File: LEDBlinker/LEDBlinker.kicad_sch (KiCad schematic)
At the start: 19 parts, among them J1 Conn_01x02_Pin, Q1 2N7000, Q2 2N7000, Q3 2N7000, SW1 SW_SPDT, U1 ICM7555xP

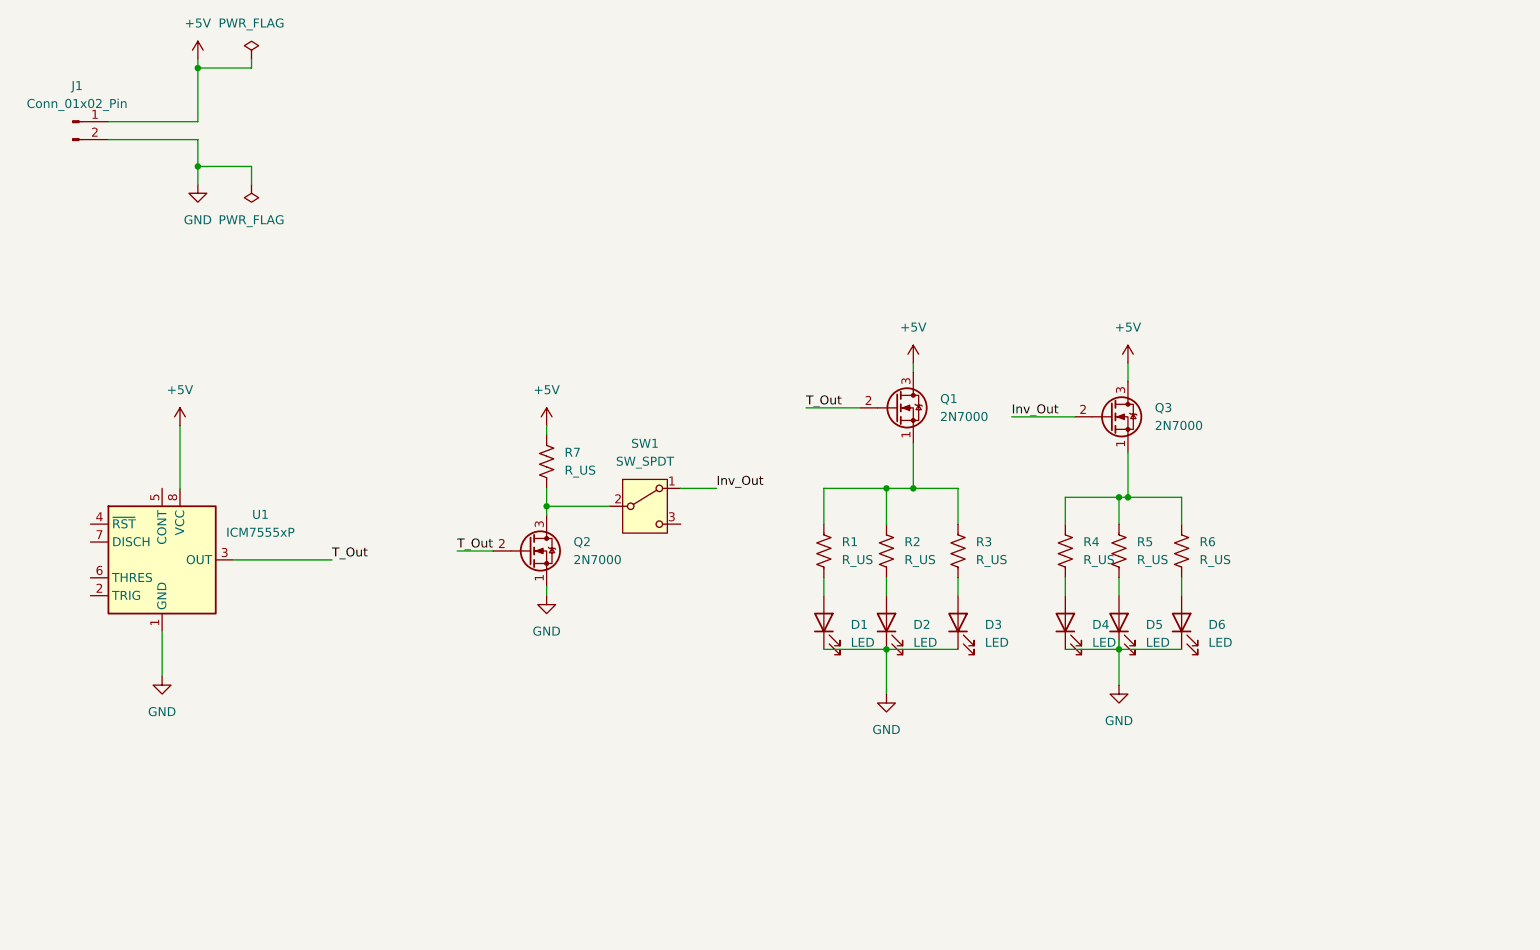
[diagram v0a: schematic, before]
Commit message: Initial Commit
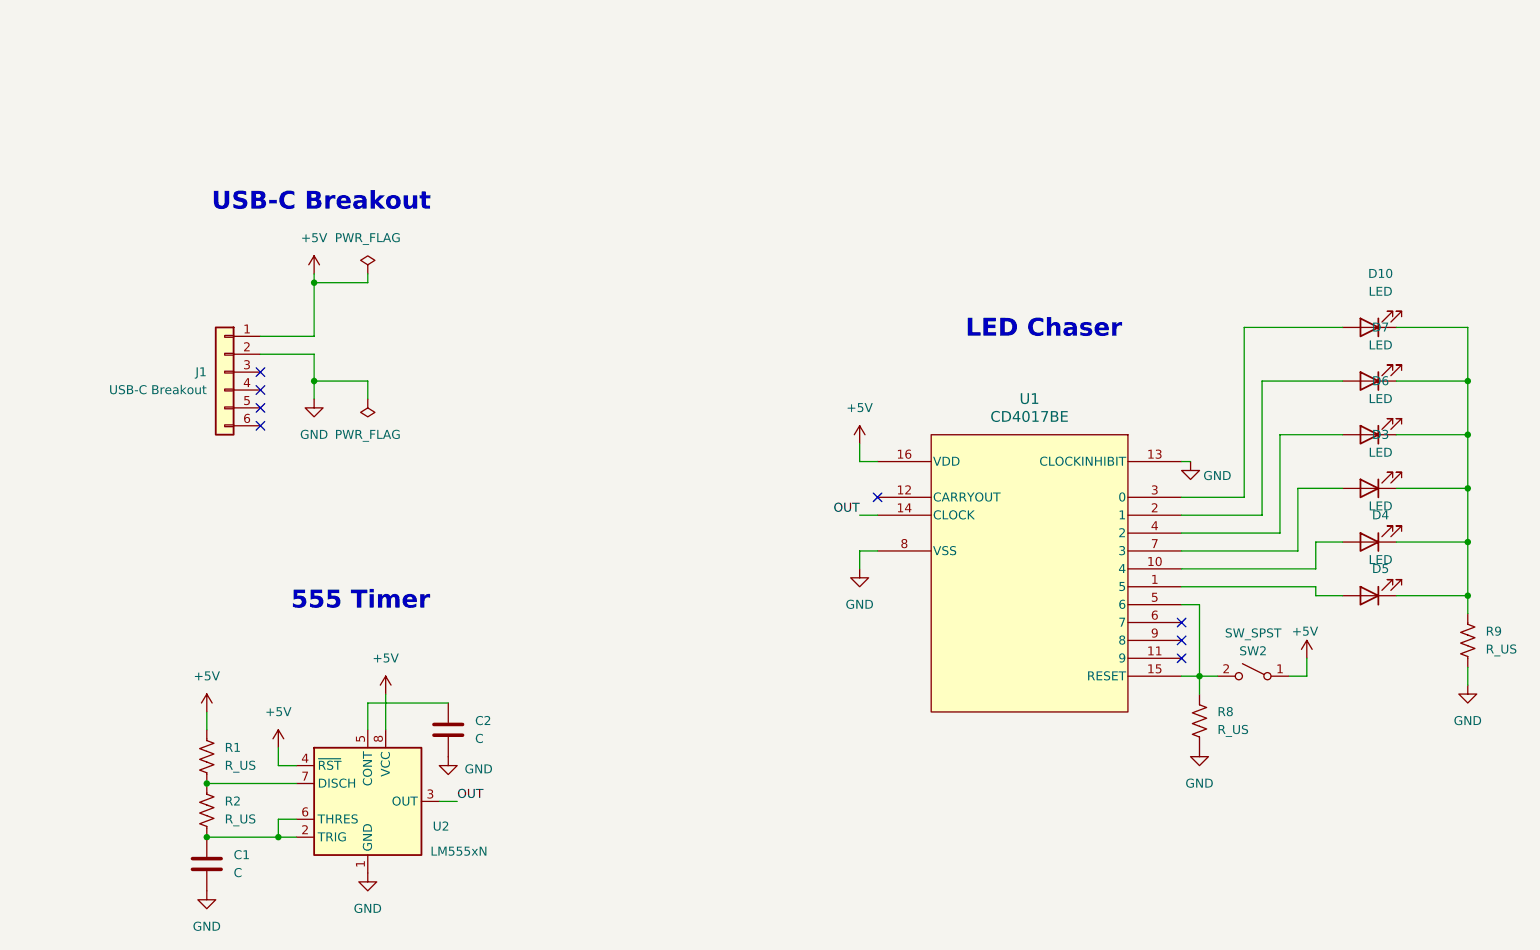
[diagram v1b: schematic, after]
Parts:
- removed D1, D2: LED, symbol Device:LED
- removed J1: Conn_01x02_Pin, symbol Connector:Conn_01x02_Pin
- removed Q1, Q2, Q3: 2N7000, Package_TO_SOT_THT:TO-92_Inline, symbol Transistor_FET:2N7000
- removed R3, R4, R5, R6, R7: R_US, symbol Device:R_US
- removed SW1: SW_SPDT, symbol Switch:SW_SPDT
- removed U1: ICM7555xP, Package_DIP:DIP-8_W7.62mm, symbol Timer:ICM7555xP
- added C1, C2: C, symbol Device:C
- added D10, D7: LED, symbol Device:LED
- added J1: USB-C Breakout, symbol Connector_Generic:Conn_01x06
- added R8, R9: R_US, symbol Device:R_US
- added SW2: SW_SPST, symbol Switch:SW_SPST
- added U1: CD4017BE, N16, symbol CD4017BE:CD4017BE
- added U2: LM555xN, Package_DIP:DIP-8_W7.62mm, symbol Timer:LM555xN
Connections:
- net +5V: now also R1.1, J1.1 (Pin_1), SW2.1 (A), U1.16 (VDD), U2.4 (~{RST}), U2.8 (VCC)
- net GND: now also C1.2, C2.2, J1.2 (Pin_2), R8.1, R9.1, U1.13 (CLOCKINHIBIT), U1.8 (VSS), U2.1 (GND); no longer D3.1 (K), D4.1 (K), D5.1 (K), D6.1 (K)
- net at D4.2 (A): now also U1.10 (4)
- net at R2.2: now also C1.1, U2.2 (TRIG), U2.6 (THRES)
- net at R2.1: now also R1.2, U2.7 (DISCH); no longer R1.1
- net at D5.2 (A): now also U1.1 (5)
- net at D3.2 (A): now also U1.7 (3)
- net at D6.2 (A): now also U1.4 (2)
- new net: D10.1 (K), D3.1 (K), D4.1 (K), D5.1 (K), D6.1 (K), D7.1 (K), R9.2
- new net: D10.2 (A), U1.3 (0)
- new net: D7.2 (A), U1.2 (1)
- new net: C2.1, U2.5 (CONT)
- new net: R8.2, SW2.2 (B), U1.15 (RESET), U1.5 (6)
- new net OUT: U1.14 (CLOCK), U2.3 (OUT)
- no-connect marks 0 -> 8
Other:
- note added: "555 Timer"
- note added: "LED Chaser"
- note added: "USB-C Breakout"
